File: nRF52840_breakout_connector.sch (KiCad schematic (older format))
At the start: 4 parts, among them J2 Conn_ARM_JTAG_SWD_10, J3 Conn_01x22, J4 Conn_01x16, J5 Conn_01x22

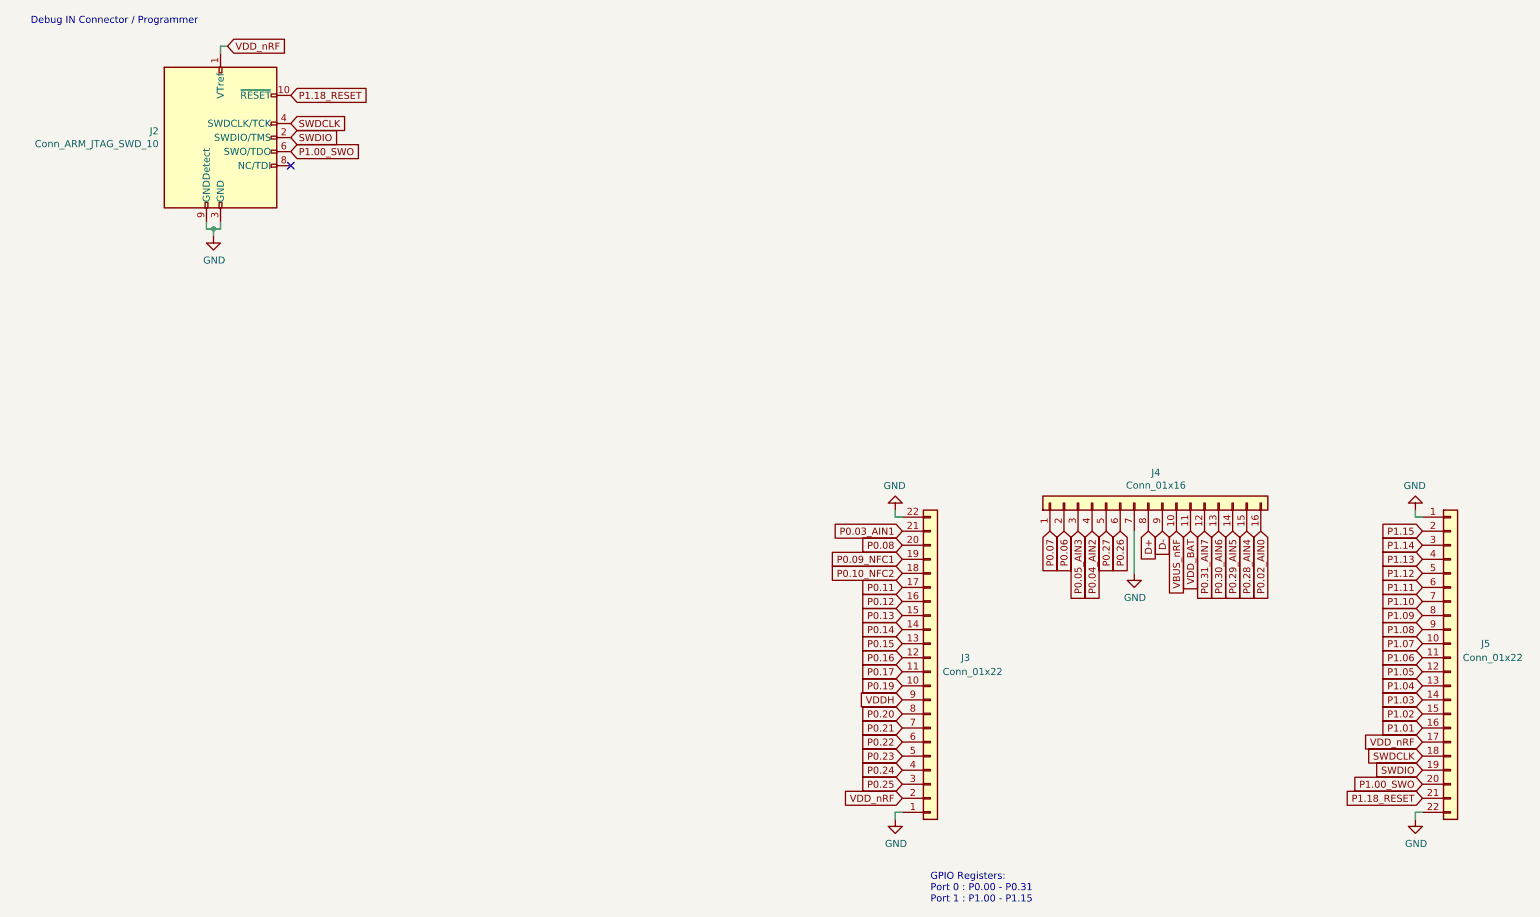
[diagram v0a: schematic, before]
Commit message: layout / added part details etc
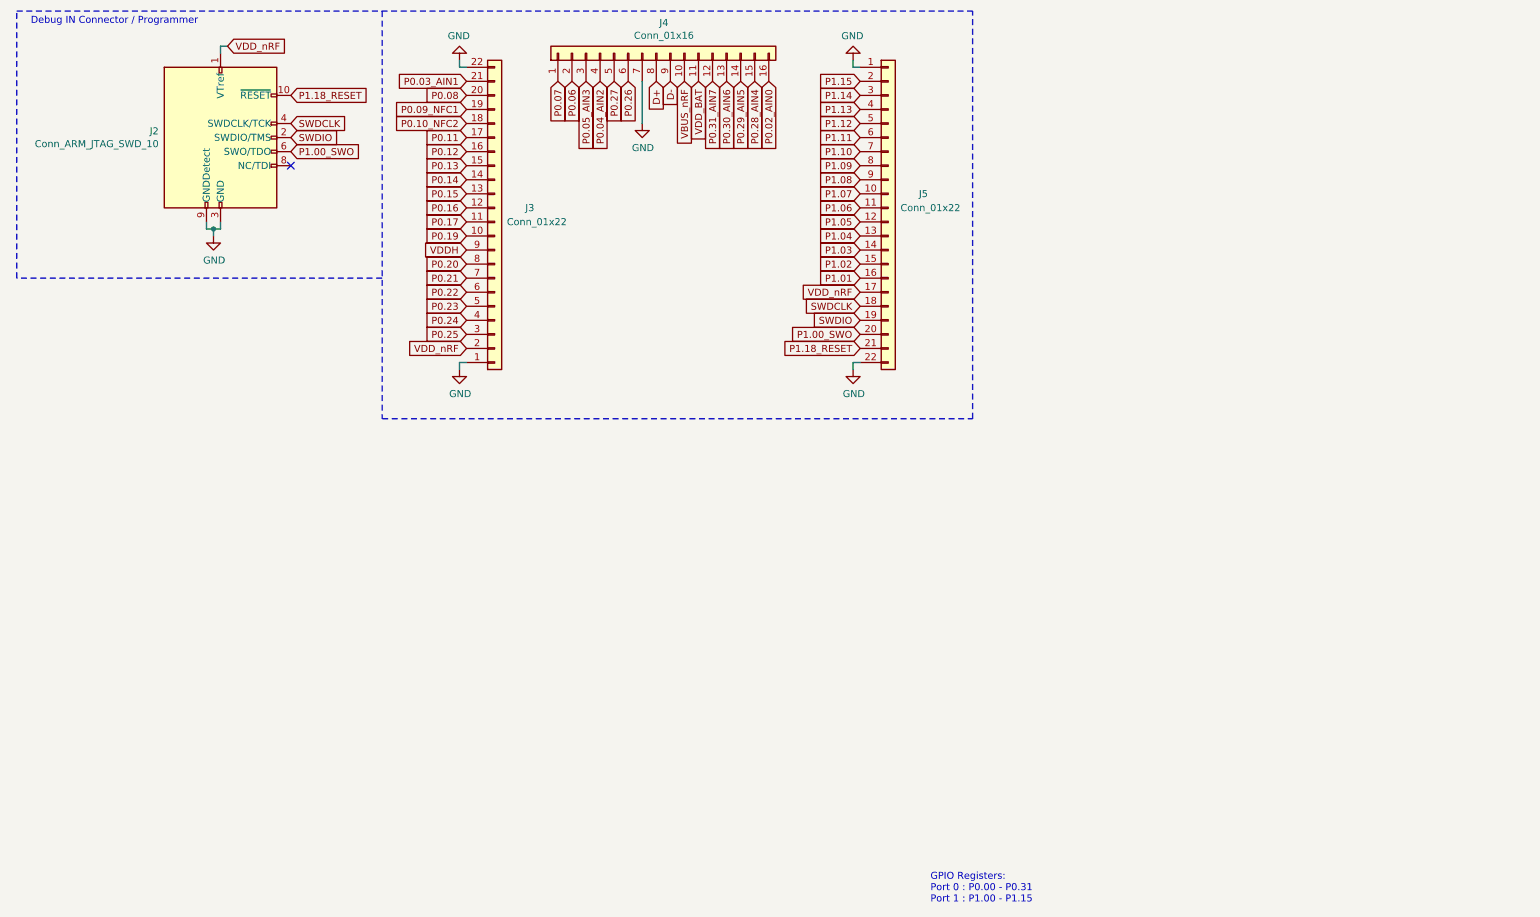
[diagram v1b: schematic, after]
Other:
- moved on the sheet: J3, J4, J5
